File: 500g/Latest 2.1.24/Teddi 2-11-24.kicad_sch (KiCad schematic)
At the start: 31 parts, among them IC1 TEENSY_4.1, J1 IR Sensor L, J10 Battery Socket, J11 IR Start Module, J2 IR Sensor R, J4 IR Sensor C, J5 Line Sensor 1, J6 Line Sensor 2, J7 Line Sensor 3, J8 Conn_01x02_Socket, J9 Conn_01x02_Socket, U1 TB67H303HG (MD), U2 TPS562200 (VR), U3 ADG3304BRUZ-REEL

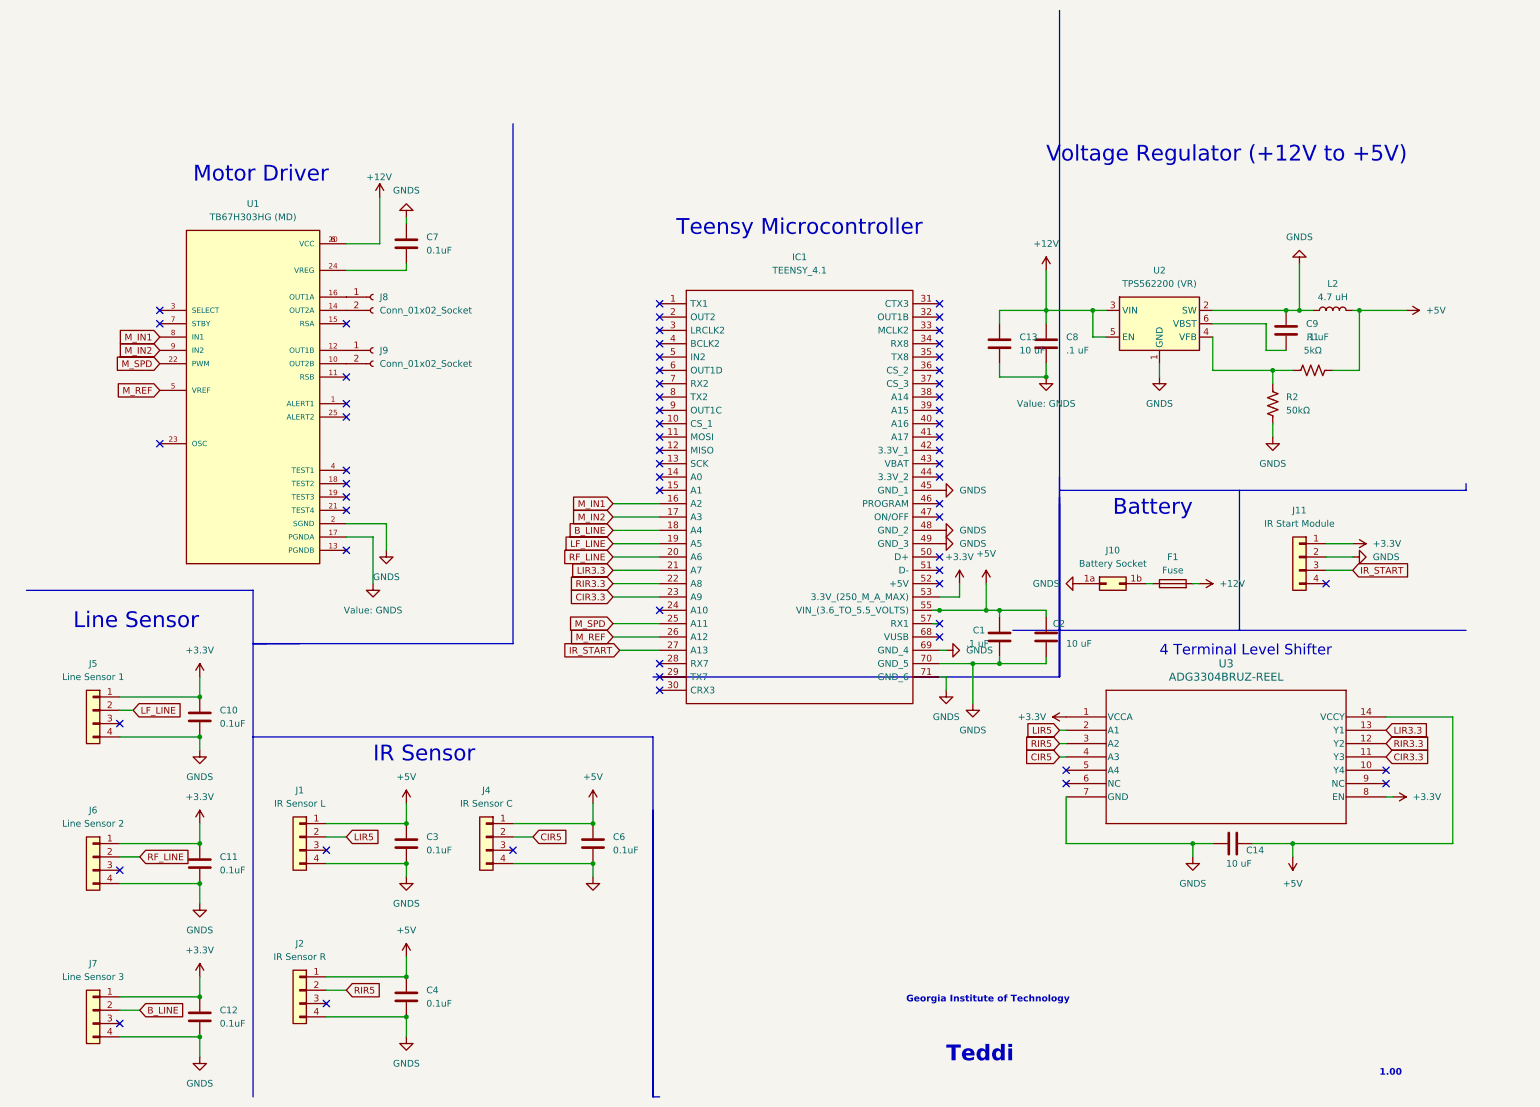
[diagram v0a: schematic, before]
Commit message: NEW Motordriver!
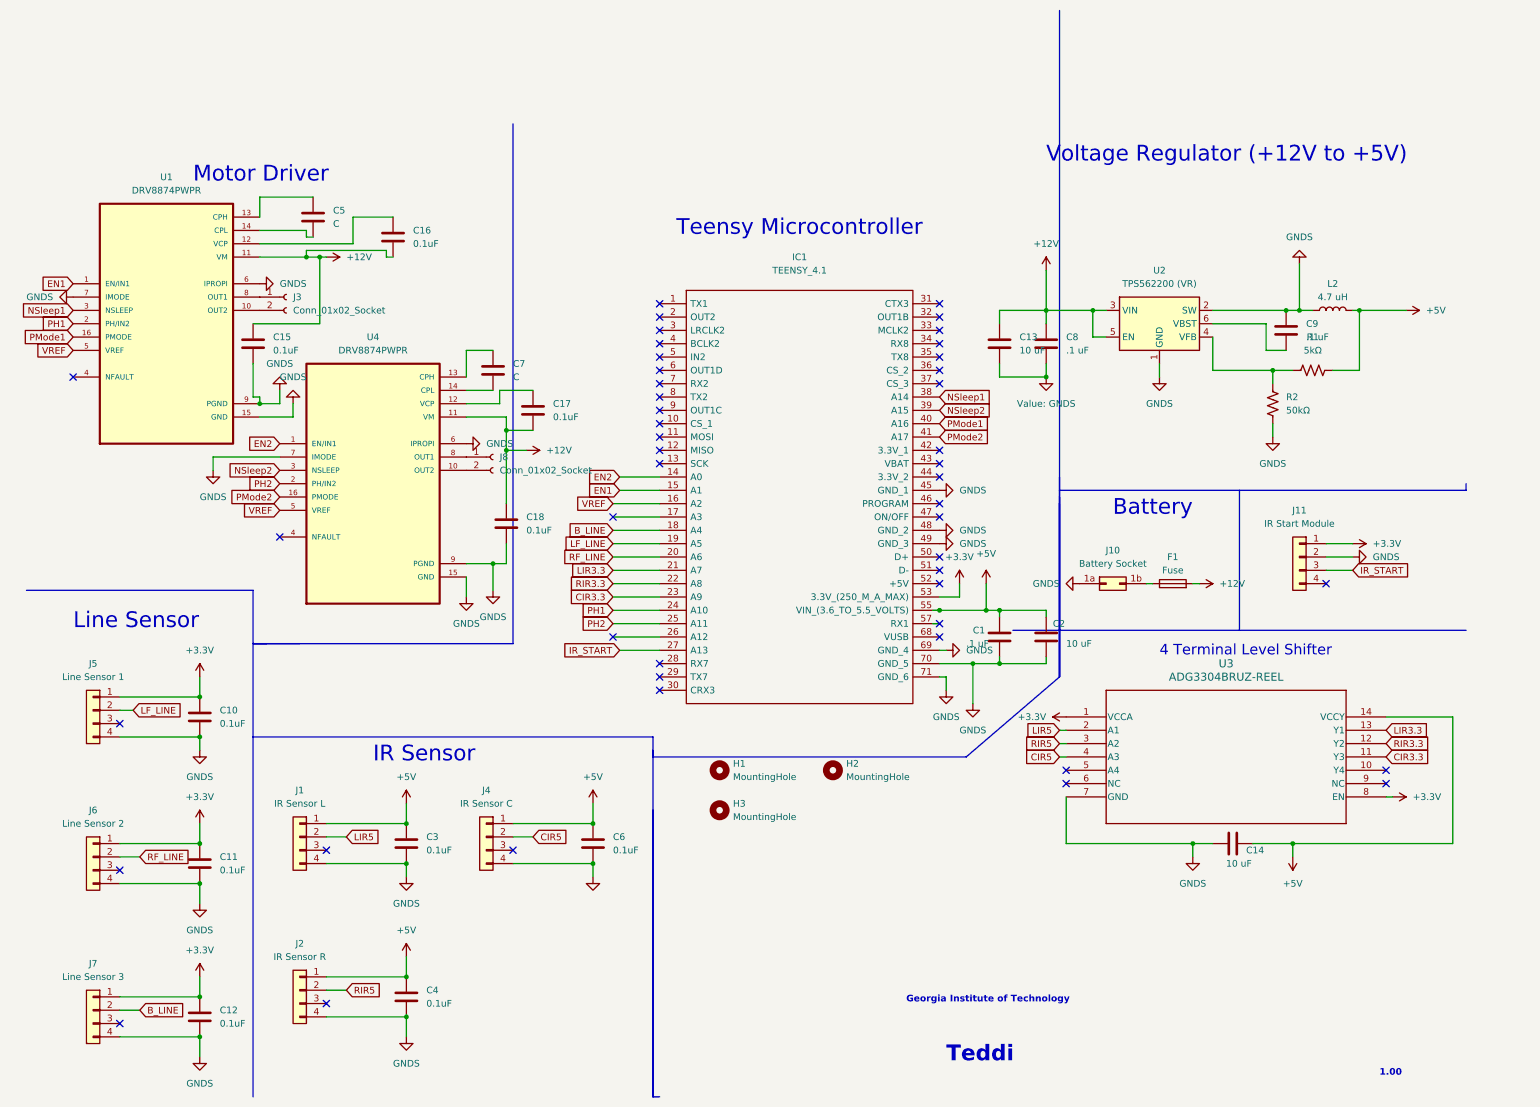
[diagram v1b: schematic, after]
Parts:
- removed J9: Conn_01x02_Socket, symbol Connector:Conn_01x02_Socket
- removed U1: TB67H303HG (MD), RoboJackets:TO100P2930X465X1937-25, symbol TB67H303HG:TB67H303HG
- added C15, C16, C17, C18: 0.1uF, Capacitor_SMD:C_0603_1608Metric, symbol Device:C
- added C5: C, Capacitor_SMD:C_0603_1608Metric, symbol Device:C
- added H1, H2, H3: MountingHole, MountingHole:MountingHole_2.1mm, symbol Mechanical:MountingHole
- added J3: Conn_01x02_Socket, Connector_PinSocket_2.54mm:PinSocket_1x02_P2.54mm_Vertical, symbol Connector:Conn_01x02_Socket
- added U1, U4: DRV8874PWPR, RoboJackets:SOP65P640X120-17N, symbol Robojackets:DRV8874PWPR
- C1, C10, C11, C12, C13, C14, C2, C3, C4, C6, C8, C9: footprint Capacitor_SMD:C_0201_0603Metric -> Capacitor_SMD:C_0603_1608Metric
- C7: value 0.1uF -> C; footprint Capacitor_SMD:C_0201_0603Metric -> Capacitor_SMD:C_0603_1608Metric
- J8: footprint (none) -> Connector_PinSocket_2.54mm:PinSocket_1x02_P2.54mm_Vertical
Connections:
- net +12V: now also C15.1, C16.2, C17.2, C18.1, U1.11 (VM), U4.11 (VM)
- net GNDS: now also C15.2, C18.2, U1.15 (GND), U1.6 (IPROPI), U1.7 (IMODE), U1.9 (PGND), U4.15 (GND), U4.6 (IPROPI), U4.7 (IMODE), U4.9 (PGND); no longer C7.1
- net at C7.2: now also U4.14 (CPL)
- net at J8.1 (Pin_1): now also U4.8 (OUT1)
- net at J8.2 (Pin_2): now also U4.10 (OUT2)
- net EN2: now reaches IC1.14 (A0)
- net EN2: now also U4.1 (EN/IN1)
- net EN1: now reaches IC1.15 (A1)
- net EN1: now also U1.1 (EN/IN1)
- net PH1: now reaches IC1.24 (A10)
- net PH1: now also U1.2 (PH/IN2)
- net NSleep1: now reaches IC1.38 (A14)
- net NSleep1: now also U1.3 (NSLEEP)
- net NSleep2: now reaches IC1.39 (A15)
- net NSleep2: now also U4.3 (NSLEEP)
- net PMode1: now reaches IC1.40 (A16)
- net PMode1: now also U1.16 (PMODE)
- net PMode2: now reaches IC1.41 (A17)
- net PMode2: now also U4.16 (PMODE)
- net M_IN1 renamed VREF
- net VREF: now also U1.5 (VREF), U4.5 (VREF)
- net M_IN2: no longer names the net of IC1.17 (A3)
- net M_REF: no longer names the net of IC1.26 (A12)
- net M_SPD renamed PH2
- net PH2: now also U4.2 (PH/IN2)
- new net: J3.2 (Pin_2), U1.10 (OUT2)
- new net: C16.1, U1.12 (VCP)
- new net: C5.1, U1.13 (CPH)
- new net: C5.2, U1.14 (CPL)
- new net: J3.1 (Pin_1), U1.8 (OUT1)
- new net: C17.1, U4.12 (VCP)
- new net: C7.1, U4.13 (CPH)
- no-connect marks 63 -> 48
